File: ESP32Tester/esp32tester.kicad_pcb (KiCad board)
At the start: 2 copper layers, 99.9 x 41.1 mm, 17 parts, among them IC1 TJA1441AT, J1 RJ45_LED_Shielded, J2 RJ45_LED_Shielded, J3 Conn_01x02_Pin, J4 Conn_01x02_Pin, J5 Screw_Terminal_01x02, U1 ESP32-DevKitC

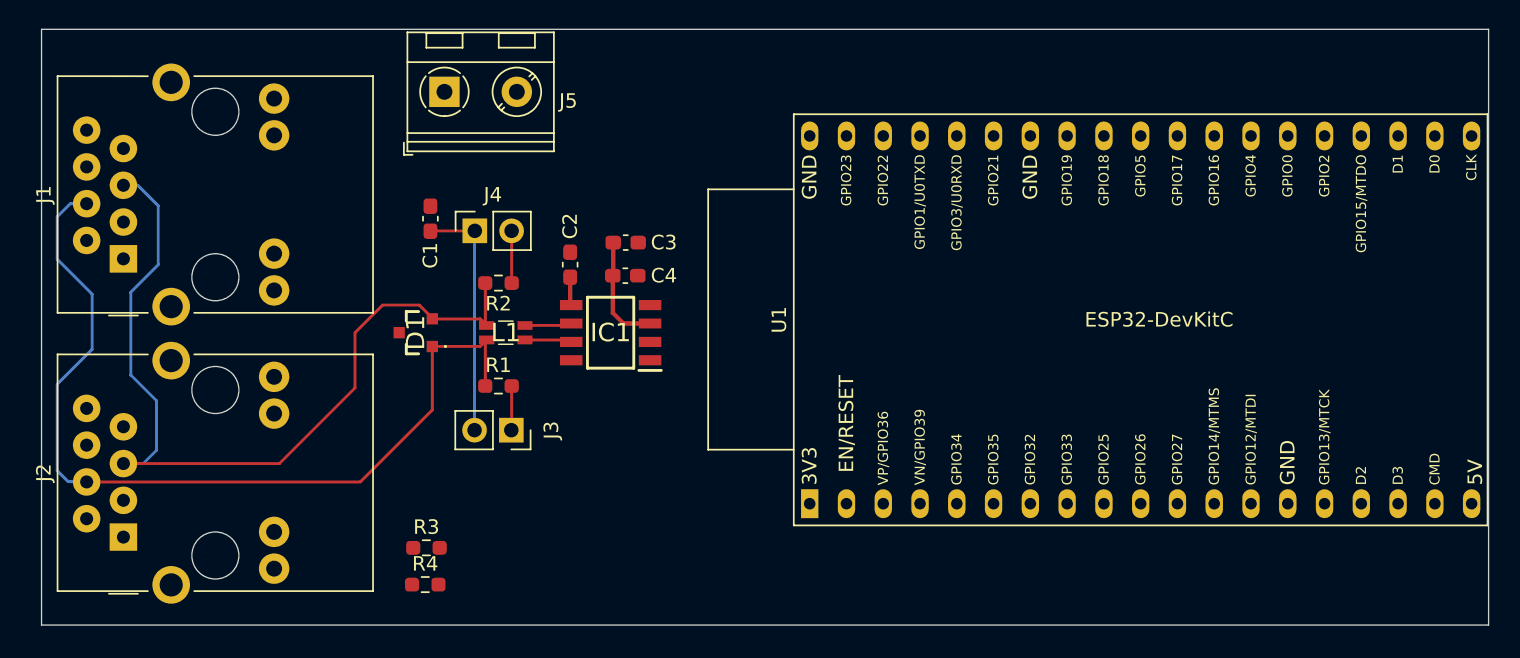
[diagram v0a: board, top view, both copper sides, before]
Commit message: 0313
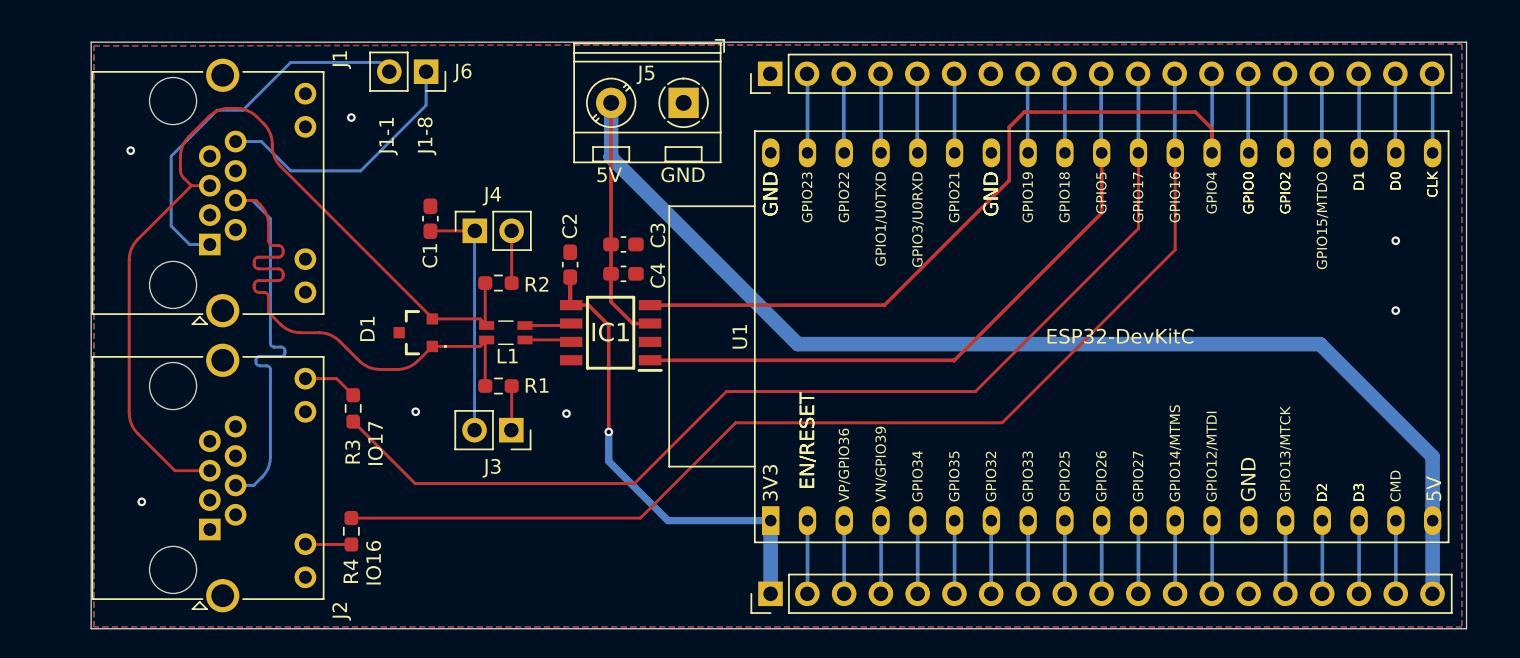
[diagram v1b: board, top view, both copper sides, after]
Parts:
- added J6: Conn_01x02_Pin, Connector_PinSocket_2.54mm:PinSocket_1x02_P2.54mm_Vertical, F.Cu at (60.0, 80.0)
- added REF**: PinHeader_1x19_P2.54mm_Vertical, Connector_PinHeader_2.54mm:PinHeader_1x19_P2.54mm_Vertical, F.Cu at (83.8, 80.2)
- added REF**: PinHeader_1x19_P2.54mm_Vertical, Connector_PinHeader_2.54mm:PinHeader_1x19_P2.54mm_Vertical, F.Cu at (83.8, 116.1)
- J1, J2: footprint Connector_RJ:RJ45_Bel_SI-60062-F -> Connector_RJ:RJ45_Amphenol_RJHSE538X
- moved J5 16.5 mm to (77.8, 82.2), turned to 180 degrees
- moved R3 10.9 mm to (55.0, 103.3), turned to -90 degrees
- moved R4 6.29 mm to (54.9, 111.8), turned to 90 degrees
- moved J1 6.05 mm to (45.1, 92.0)
- moved J2 5.99 mm to (45.1, 111.6)
- moved U1 2.93 mm to (83.8, 111.0)
- moved C3 0.20 mm to (73.7, 91.9)
- moved C4 0.18 mm to (73.7, 94.0)
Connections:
- net Net-(D1-Pad1) renamed /CAN_BUS+
- net Net-(D1-Pad2) renamed /CAN_BUS-
- net Net-(IC1-RXD) renamed GPIO4
- net Net-(IC1-TXD) renamed GPIO5
- J1 pad 1: unconnected-(J1-Pad1) -> Net-(J6-Pin_2)
- J1 pad 8: unconnected-(J1-Pad8) -> Net-(J6-Pin_1)
- R3 pad 2: Net-(U1-GPIO16) -> GPIO17
- R4 pad 2: Net-(U1-GPIO17) -> GPIO16
- U1 pad 2: unconnected-(U1-CHIP_PU-Pad2) -> reset
- U1 pad 20: unconnected-(U1-SD_CLK/GPIO6-Pad20) -> clk
- U1 pad 21: unconnected-(U1-SD_DATA0/GPIO7-Pad21) -> D0
- U1 pad 22: unconnected-(U1-SD_DATA1/GPIO8-Pad22) -> D1
- U1 pad 23: unconnected-(U1-MTDO/GPIO15/ADC2_CH3-Pad23) -> GPIO15
- U1 pad 24: unconnected-(U1-ADC2_CH2/GPIO2-Pad24) -> GPIO2
- U1 pad 25: unconnected-(U1-GPIO0/BOOT/ADC2_CH1-Pad25) -> GPIO0
- U1 pad 27: Net-(U1-GPIO16) -> GPIO16
- U1 pad 28: Net-(U1-GPIO17) -> GPIO17
- U1 pad 3: unconnected-(U1-SENSOR_VP/GPIO36/ADC1_CH0-Pad3) -> GPIO36
- U1 pad 30: unconnected-(U1-GPIO18-Pad30) -> GPIO18
- U1 pad 31: unconnected-(U1-GPIO19-Pad31) -> GPIO19
- U1 pad 33: unconnected-(U1-GPIO21-Pad33) -> GPIO21
- U1 pad 34: unconnected-(U1-U0RXD/GPIO3-Pad34) -> GPIO3
- U1 pad 35: unconnected-(U1-U0TXD/GPIO1-Pad35) -> GPIO1
- U1 pad 36: unconnected-(U1-GPIO22-Pad36) -> GPIO22
- U1 pad 37: unconnected-(U1-GPIO23-Pad37) -> GPIO23
- U1 pad 4: unconnected-(U1-SENSOR_VN/GPIO39/ADC1_CH3-Pad4) -> GPIO39
- U1 pad 5: unconnected-(U1-VDET_1/GPIO34/ADC1_CH6-Pad5) -> GPIO34
- U1 pad 6: unconnected-(U1-VDET_2/GPIO35/ADC1_CH7-Pad6) -> GPIO35
- U1 pad 7: unconnected-(U1-32K_XP/GPIO32/ADC1_CH4-Pad7) -> GPIO32
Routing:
- net Net-(IC1-VCC): track 7.74 -> 95.6 mm
- net GPIO16: track 0.00 -> 76.8 mm
- net GPIO17: track 0.00 -> 74.0 mm
- net GPIO4: track 0.00 -> 54.1 mm
- net GPIO5: track 0.00 -> 45.1 mm
- net Net-(IC1-VIO): track 1.96 -> 32.5 mm, vias 0 -> 1
- net Net-(J6-Pin_2): track 0.00 -> 26.0 mm
- net Net-(J6-Pin_1): track 0.00 -> 18.2 mm
- net D0: track 0.00 -> 5.48 mm
- net clk: track 0.00 -> 5.48 mm
- net GPIO23: track 0.00 -> 5.48 mm
- net GPIO18: track 0.00 -> 5.48 mm
- net GPIO1: track 0.00 -> 5.48 mm
- net D1: track 0.00 -> 5.48 mm
- net GPIO3: track 0.00 -> 5.48 mm
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- added copper zone on B.Cu, net GND
- added copper zone on F.Cu, net GND
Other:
- board size 99.9 x 41.1 mm -> 95 x 40.5 mm
- board text added: "3V3"
- board text added: "5V"
- board text added: "CAN H"
- board text added: "CAN L"
- board text added: "CLK"
- board text added: "CMD"
- board text added: "D0"
- board text added: "D1"
- board text added: "D2"
- board text added: "D3"
- board text added: "EN/RESET"
- board text added: "GND"
- board text added: "GPIO0"
- board text added: "GPIO1/U0TXD"
- board text added: "GPIO12/MTDI"
- board text added: "GPIO13/MTCK"
- board text added: "GPIO14/MTMS"
- board text added: "GPIO15/MTDO"
- board text added: "GPIO16"
- board text added: "GPIO17"
- board text added: "GPIO18"
- board text added: "GPIO19"
- board text added: "GPIO2"
- board text added: "GPIO21"
- board text added: "GPIO22"
- board text added: "GPIO23"
- board text added: "GPIO25"
- board text added: "GPIO26"
- board text added: "GPIO27"
- board text added: "GPIO3/U0RXD"
- board text added: "GPIO32"
- board text added: "GPIO33"
- board text added: "GPIO34"
- board text added: "GPIO35"
- board text added: "GPIO4"
- board text added: "GPIO5"
- board text added: "IO16"
- board text added: "IO17"
- board text added: "J1"
- board text added: "J1-1"
- board text added: "J1-8"
- board text added: "J2"
- board text added: "J5"
- board text added: "VN/GPIO39"
- board text added: "VP/GPIO36"
